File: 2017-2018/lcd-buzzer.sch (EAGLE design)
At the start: 12 parts, among them J1 AVR_SPI_PROG2PTH2, U1 ATMEGA328P-MUR, U2 DRV2605YZFR, U3 74HC595PW, U4 74HC595PW, U5 74HC595PW, U6 74HC595PW

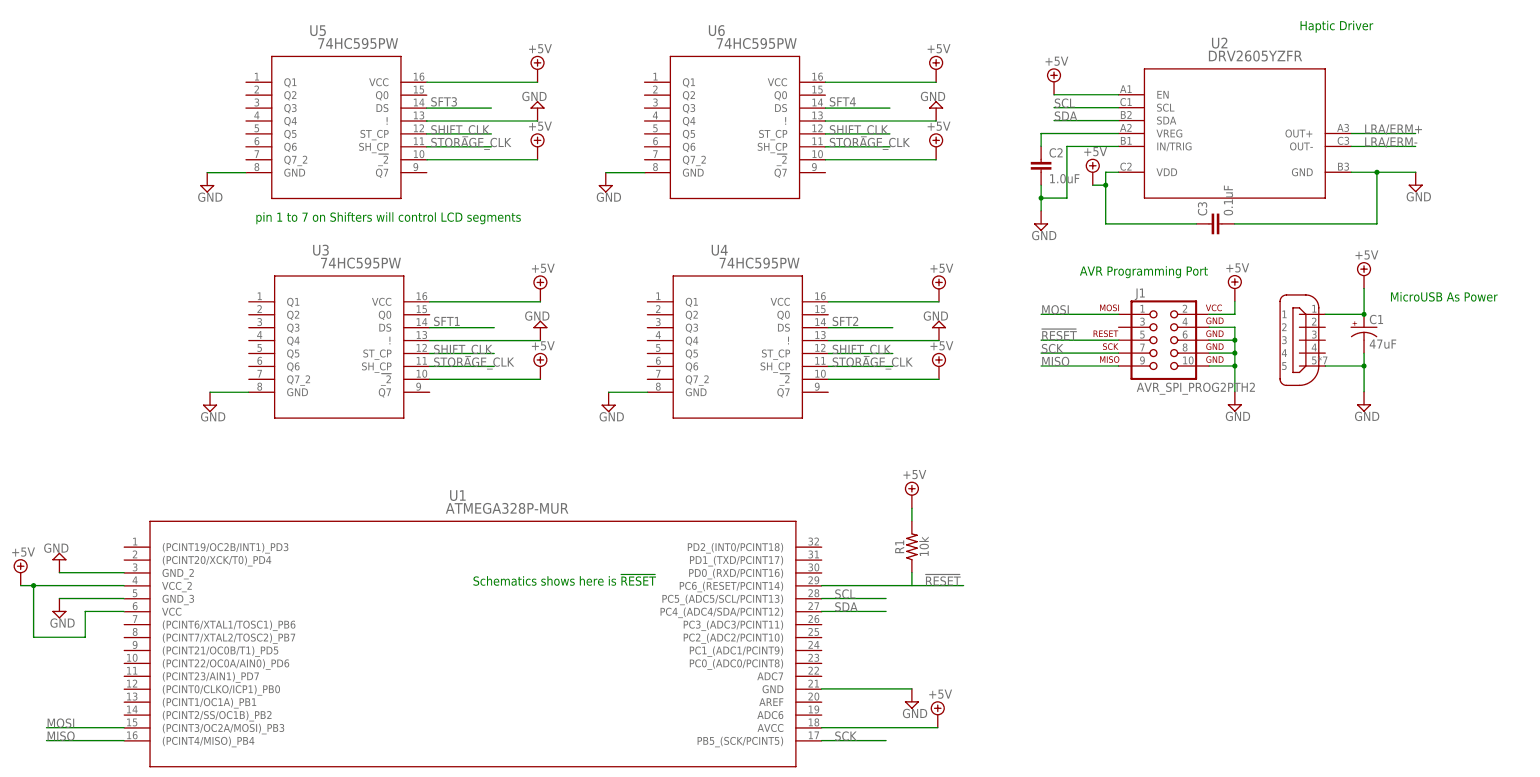
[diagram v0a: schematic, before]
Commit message: First Version Completed
Added extra custom parts to the library, completed the schematics
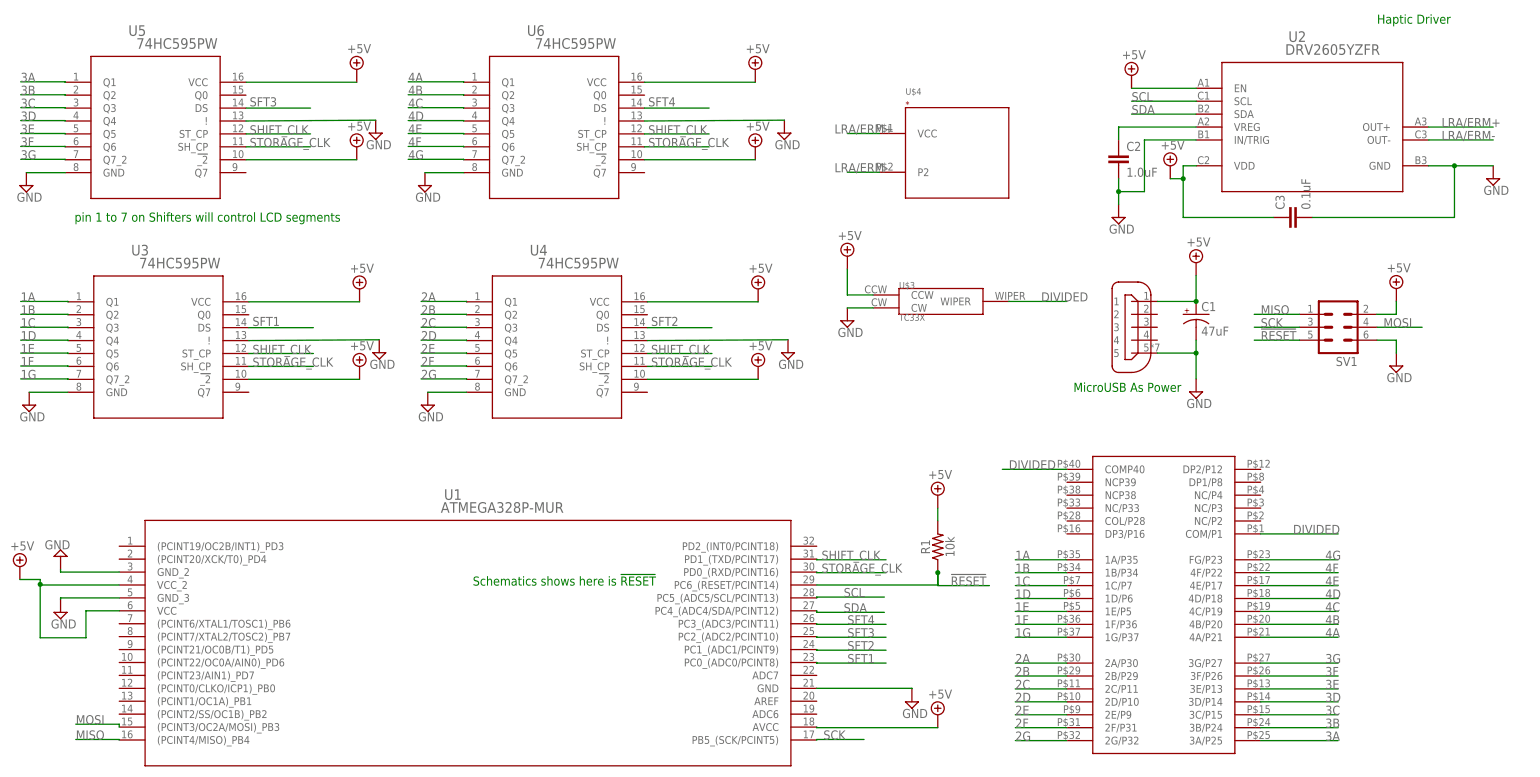
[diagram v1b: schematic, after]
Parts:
- removed J1: AVR_SPI_PROG2PTH2, rgb-led:AVR_SPI_PROG2PTH2
- added SV1: (no value), con-lstb:MA03-2
- added U$2: LCD-S401C39TR, lcd-buzzer:LCD-S401C39TR
- added U$3: TC33X, lcd-buzzer:TC33X
- added U$4: PS1240P02BT, lcd-buzzer:PS1240P02BT
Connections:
- new net 1A: U$2.1A/P35, U3.Q1
- new net 1B: U$2.1B/P34, U3.Q2
- new net 1C: U$2.1C/P7, U3.Q3
- new net 1D: U$2.1D/P6, U3.Q4
- new net 1E: U$2.1E/P5, U3.Q5
- new net 1F: U$2.1F/P36, U3.Q6
- new net 1G: U$2.1G/P37, U3.Q7_2
- new net 2A: U$2.2A/P30, U4.Q1
- new net 2B: U$2.2B/P29, U4.Q2
- new net 2C: U$2.2C/P11, U4.Q3
- new net 2D: U$2.2D/P10, U4.Q4
- new net 2E: U$2.2E/P9, U4.Q5
- new net 2F: U$2.2F/P31, U4.Q6
- new net 2G: U$2.2G/P32, U4.Q7_2
- new net 3A: U$2.3A/P25, U5.Q1
- new net 3B: U$2.3B/P24, U5.Q2
- new net 3C: U$2.3C/P15, U5.Q3
- new net 3D: U$2.3D/P14, U5.Q4
- new net 3E: U$2.3E/P13, U5.Q5
- new net 3F: U$2.3F/P26, U5.Q6
- new net 3G: U$2.3G/P27, U5.Q7_2
- new net 4A: U$2.4A/P21, U6.Q1
- new net 4B: U$2.4B/P20, U6.Q2
- new net 4C: U$2.4C/P19, U6.Q3
- new net 4D: U$2.4D/P18, U6.Q4
- new net 4E: U$2.4E/P17, U6.Q5
- new net 4F: U$2.4F/P22, U6.Q6
- new net 4G: U$2.FG/P23, U6.Q7_2
- new net DIVIDED: U$2.COM/P1, U$2.COMP40, U$3.WIPER
- net !RESET: now also SV1.5, U1.PC6_(RESET/PCINT14); no longer J1.RESET
- net +5V: now also SV1.2, U$3.CCW, U1.AVCC, U1.VCC, U1.VCC_2; no longer J1.VCC
- net GND: now also SV1.6, U$3.CW, U1.GND, U1.GND_2, U1.GND_3; no longer J1.GND@1, J1.GND@2, J1.GND@3, J1.GND@4
- net LRA/ERM+: now also U$4.VCC
- net LRA/ERM-: now also U$4.P2
- net MISO: now also SV1.1, U1.(PCINT4/MISO)_PB4; no longer J1.MISO
- net MOSI: now also SV1.4, U1.(PCINT3/OC2A/MOSI)_PB3; no longer J1.MOSI
- net SCK: now also SV1.3, U1.PB5_(SCK/PCINT5); no longer J1.SCK
- net SCL: now also U1.PC5_(ADC5/SCL/PCINT13)
- net SDA: now also U1.PC4_(ADC4/SDA/PCINT12)
- net SFT1: now also U1.PC0_(ADC0/PCINT8)
- net SFT2: now also U1.PC1_(ADC1/PCINT9)
- net SFT3: now also U1.PC2_(ADC2/PCINT10)
- net SFT4: now also U1.PC3_(ADC3/PCINT11)
- net SHIFT_CLK: now also U1.PD1_(TXD/PCINT17)
- net STORAGE_CLK: now also U1.PD0_(RXD/PCINT16)
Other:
- note removed: "AVR Programming Port"
- moved on the sheet: C1, C2, C3, R1, U1, U2, U3, U4, U5, U6
